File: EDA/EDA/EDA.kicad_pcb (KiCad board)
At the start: 2 copper layers, 26 parts, among them J1 EXT_INTF, J2 EXT_BOOT, J3 XM132_SWD, U1 ATmega328PB-MU, U2 74AHC126BQ, U3 MIC94091YC6, U4 KXTJ3-1057, Y1 8 MHz

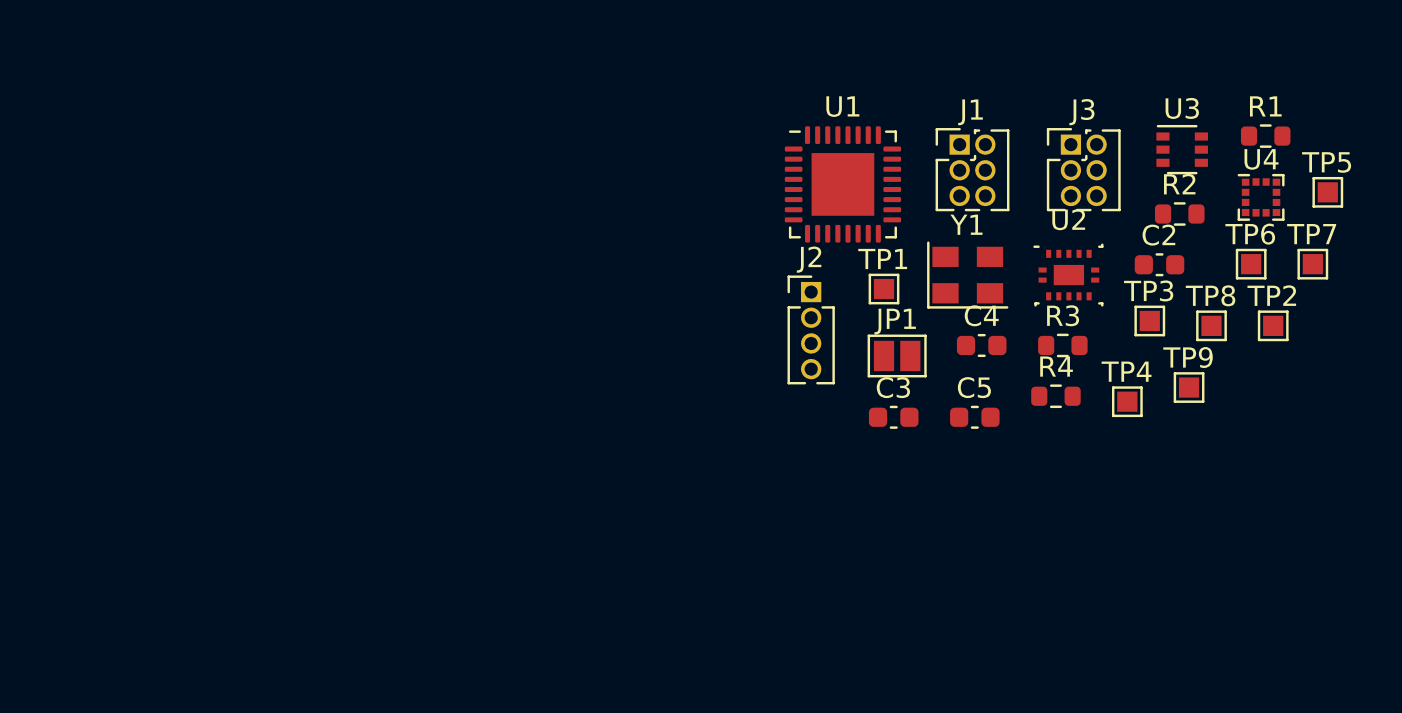
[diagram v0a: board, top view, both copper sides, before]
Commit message: more work on PCB routing
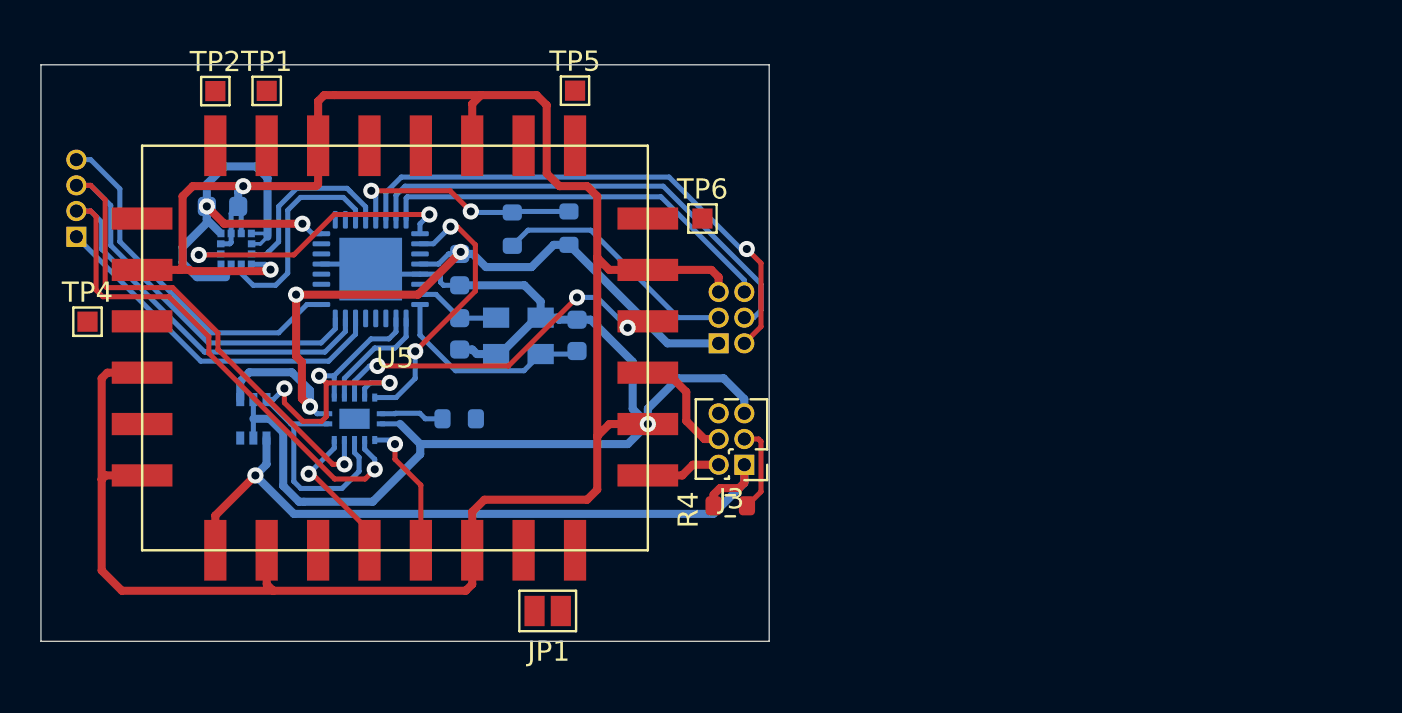
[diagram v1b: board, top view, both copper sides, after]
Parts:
- removed TP3: 1V8_OUT, TestPoint:TestPoint_Pad_1.0x1.0mm
- removed TP7: MISC_GPIO0, TestPoint:TestPoint_Pad_1.0x1.0mm
- removed TP8: MISC_GPIO1, TestPoint:TestPoint_Pad_1.0x1.0mm
- removed TP9: MISC_GPIO2, TestPoint:TestPoint_Pad_1.0x1.0mm
- added U5: XM132, EDA:XM132, F.Cu at (100.0, 100.0)
- C2, C3, C4, C5, J1, J2, R1, R2, R3, U1, U2, U3, U4, Y1: moved to B.Cu
- moved TP2 53.6 mm to (91.1, 87.3)
- moved TP4 51.6 mm to (84.8, 98.7)
- moved U4 50.7 mm to (92.2, 95.1), turned to 90 degrees
- moved U3 47.8 mm to (93.0, 103.5), turned to 90 degrees
- moved C5 38.6 mm to (91.5, 93.0)
- moved TP5 37.6 mm to (108.9, 87.3)
- moved J2 36.4 mm to (84.2, 94.5)
- moved U2 36.0 mm to (98.0, 103.5)
- moved R1 34.7 mm to (108.6, 94.1), turned to 90 degrees
- moved C2 34.6 mm to (103.2, 96.1), turned to 270 degrees
- moved R2 33.0 mm to (105.8, 94.1), turned to 90 degrees
- moved TP1 32.0 mm to (93.7, 87.3)
- moved R3 30.1 mm to (103.2, 103.5), turned to 180 degrees
- moved TP6 27.2 mm to (115.2, 93.6)
- moved C4 25.8 mm to (103.2, 99.3), turned to 270 degrees
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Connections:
- U1 pad 11: VACC -> Net-(U1-Pad11)
- U1 pad 24: Net-(U1-Pad24) -> VACC
- U1 pad 7: Net-(U1-Pad7) -> Net-(C4-Pad1)
- U1 pad 8: Net-(U1-Pad8) -> Net-(C3-Pad1)
- U2 pad 2: MOSI -> RDR_RX
- U2 pad 3: RDR_TX -> MISO
- U2 pad 5: RDR_RX -> MOSI
- U2 pad 6: MISO -> RDR_TX
- Y1 pad 1: Net-(U1-Pad7) -> Net-(C4-Pad1)
- Y1 pad 2: Net-(C4-Pad1) -> GND
- Y1 pad 3: Net-(U1-Pad8) -> Net-(C3-Pad1)
- Y1 pad 4: Net-(C3-Pad1) -> GND
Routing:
- net GND: track 0.00 -> 180.5 mm, vias 0 -> 3
- net MOSI: track 0.00 -> 42.7 mm, vias 0 -> 1
- net MISO: track 0.00 -> 41.1 mm, vias 0 -> 1
- net +3V3: track 0.00 -> 40.6 mm, vias 0 -> 3
- net VRDR: track 0.00 -> 36.3 mm, vias 0 -> 1
- net VRDR_EN: track 0.00 -> 29.7 mm, vias 0 -> 3
- net TTL_RX: track 0.00 -> 26.3 mm, vias 0 -> 1
- net VACC: track 0.00 -> 25.3 mm, vias 0 -> 2
- net TTL_TX: track 0.00 -> 23.7 mm
- net TTL_WKE: track 0.00 -> 20.1 mm
- net RDR_WKE: track 0.00 -> 17.8 mm, vias 0 -> 3
- net SCLK: track 0.00 -> 17.8 mm
- net SS: track 0.00 -> 17.7 mm
- net ACC_INT: track 0.00 -> 14.5 mm, vias 0 -> 2
- net Net-(U1-Pad2): track 0.00 -> 13.7 mm, vias 0 -> 2
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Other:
- board outline added: 36 x 28.5 mm
- rule trace_min: 0.2 -> 0.155
